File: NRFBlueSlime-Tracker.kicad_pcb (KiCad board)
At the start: 4 copper layers, 30 x 23.5 mm, 81 parts, among them J1 HC-TYPE-C-16P-C10B, Q1 YFW2301T, SW1 TS-1088-AR02016, U1 nRF52840, U2 NPM1100-QDAA-R, U3 ICM-45686, U4 LIS2MDL, X1 SX2M32.768KM20F30TNN, Y1 XL7EL89CKI-111YLC-32M

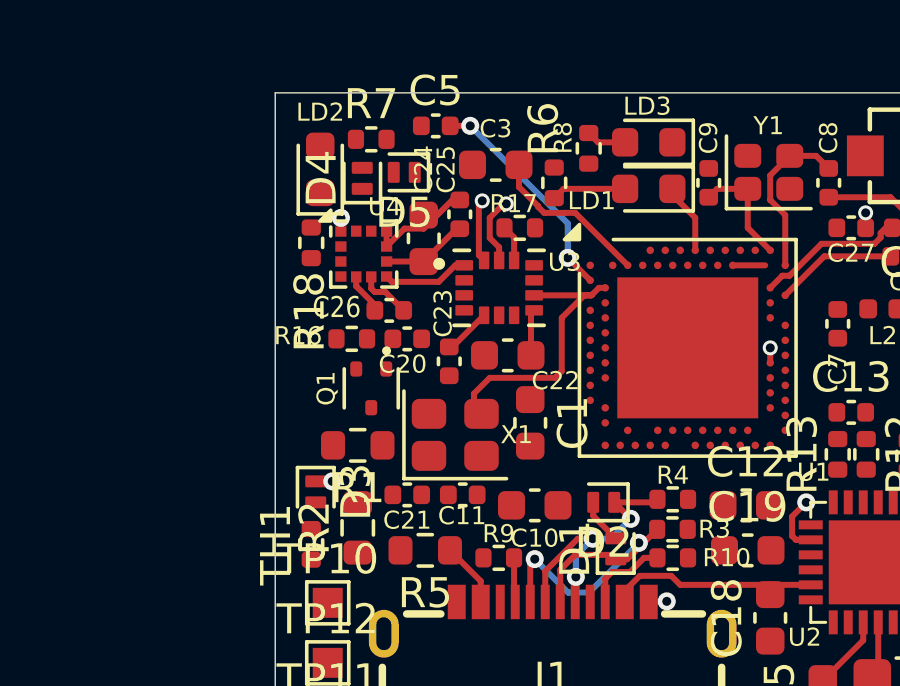
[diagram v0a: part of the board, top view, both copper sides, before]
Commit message: sync
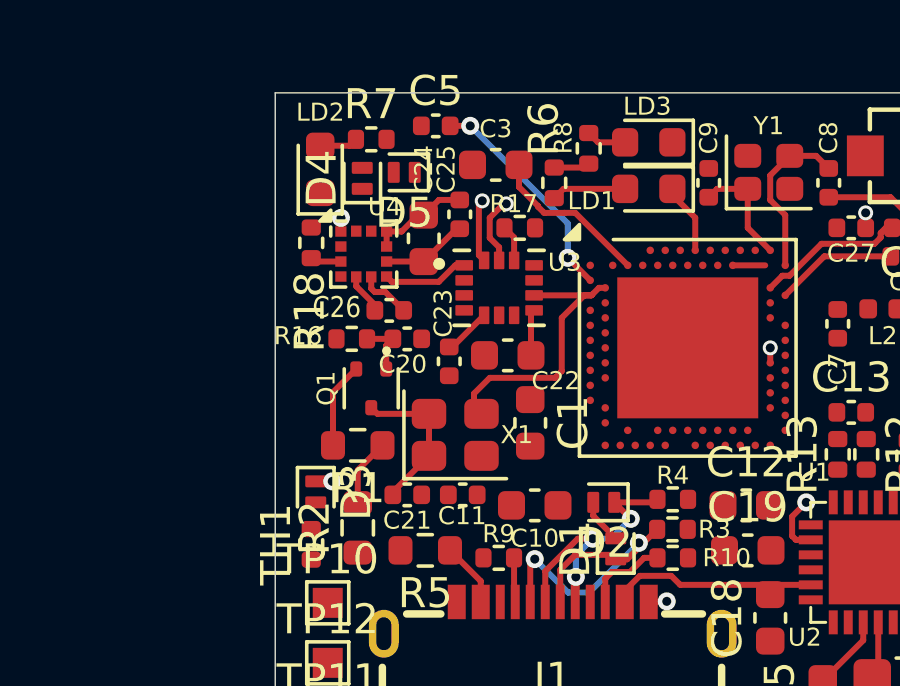
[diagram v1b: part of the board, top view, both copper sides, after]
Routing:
- net Net-(Q1-D): track 0.00 -> 5.21 mm
- net +1V8: track 10.4 -> 14.2 mm
- net Net-(U1-VDDH): track 0.00 -> 2.27 mm
- net ~{OSC_EN}: track 0.00 -> 1.96 mm
- net Net-(LD2-A): track 0.00 -> 1.28 mm
- net ~{CS}_MAG: track 0.00 -> 1.03 mm
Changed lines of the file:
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@@
+	)
+	(segment
+		(start 87.5625 47.1225)
+		(end 88.4375 47.1225)
+		(width 0.2)
+		(layer "F.Cu")
+		(net 21)
+	)
+	(segment
+		(start 87.45 47.01)
+		(end 87.5625 47.1225)
+		(width 0.2)
+		(layer "F.Cu")
+		(net 21)
 	)
 	(segment
@@
 	)
 	(segment
+		(start 92.4 45.07)
+		(end 91.705 45.07)
+		(width 0.2)
+		(layer "F.Cu")
+		(net 33)
+	)
+	(segment
 		(start 92.1575 49.97)
 		(end 93.2125 48.915)
@@
 	)
 	(segment
+		(start 96.57 43.99)
+		(end 96.7 43.86)
+		(width 0.2)
+		(layer "F.Cu")
+		(net 33)
+	)
+	(segment
 		(start 92.05 49.97)
 		(end 92.1575 49.97)
@@
 	)
 	(segment
+		(start 91.705 45.07)
+		(end 91.2 45.575)
+		(width 0.2)
+		(layer "F.Cu")
+		(net 33)
+	)
+	(segment
 		(start 89.9625 46.1225)
 		(end 89.9625 46.6225)
@@
 	)
 	(segment
-		(start 92.4 45.07)
-		(end 92.155 45.07)
-		(width 0.2)
-		(layer "F.Cu")
-		(net 33)
-	)
-	(segment
-		(start 92.155 45.07)
-		(end 91.2 46.025)
-		(width 0.2)
-		(layer "F.Cu")
-		(net 33)
-	)
-	(segment
 		(start 94.775 48.8525)
 		(end 94.8775 48.75)
@@
 	)
 	(segment
-		(start 90.56 46.025)
-		(end 89.9625 46.6225)
-		(width 0.2)
-		(layer "F.Cu")
-		(net 33)
-	)
-	(segment
-		(start 91.2 46.025)
-		(end 90.56 46.025)
+		(start 88.175 53.25)
+		(end 88.175 51.48)
+		(width 0.2)
+		(layer "F.Cu")
+		(net 33)
+	)
+	(segment
+		(start 95.55 43.99)
+		(end 96.57 43.99)
+		(width 0.2)
+		(layer "F.Cu")
+		(net 33)
+	)
+	(segment
+		(start 91.01 45.575)
+		(end 90.4625 46.1225)
+		(width 0.2)
+		(layer "F.Cu")
+		(net 33)
+	)
+	(segment
+		(start 91.2 45.575)
+		(end 91.01 45.575)
+		(width 0.2)
+		(layer "F.Cu")
+		(net 33)
+	)
+	(segment
+		(start 90.4625 46.1225)
+		(end 89.9625 46.1225)
 		(width 0.2)
 		(layer "F.Cu")
@@
 	)
 	(segment
+		(start 88.175 51.48)
+		(end 88.95 50.705)
+		(width 0.2)
+		(layer "F.Cu")
+		(net 33)
+	)
+	(segment
 		(start 101.61 64)
 		(end 101.13 63.52)
@@
 	)
 	(segment
+		(start 89.95 49.92)
+		(end 90.17 49.7)
+		(width 0.2)
+		(layer "F.Cu")
+		(net 38)
+	)
+	(segment
+		(start 89.95 50.705)
+		(end 89.95 49.92)
+		(width 0.2)
+		(layer "F.Cu")
+		(net 38)
+	)
+	(segment
+		(start 89.31 49.7)
+		(end 90.17 49.7)
+		(width 0.2)
+		(layer "F.Cu")
+		(net 38)
+	)
+	(segment
+		(start 91.375 52.2)
+		(end 89.655 52.2)
+		(width 0.2)
+		(layer "F.Cu")
+		(net 42)
+	)
+	(segment
+		(start 90.17 54.805)
+		(end 91.375 53.6)
+		(width 0.2)
+		(layer "F.Cu")
+		(net 42)
+	)
+	(segment
+		(start 90.17 54.9)
+		(end 90.17 54.805)
+		(width 0.2)
+		(layer "F.Cu")
+		(net 42)
+	)
+	(segment
+		(start 91.375 53.6)
+		(end 91.375 52.2)
+		(width 0.2)
+		(layer "F.Cu")
+		(net 42)
+	)
+	(segment
+		(start 89.655 52.2)
+		(end 89.45 51.995)
+		(width 0.2)
+		(layer "F.Cu")
+		(net 42)
+	)
+	(segment
 		(start 89.651822 48.65)
 		(end 88.95 47.948178)
@@
 	)
 	(segment
+		(start 88.7275 43.2625)
+		(end 88.94 43.05)
+		(width 0.2)
+		(layer "F.Cu")
+		(net 72)
+	)
+	(segment
+		(start 87.75 43.2625)
+		(end 88.7275 43.2625)
+		(width 0.2)
+		(layer "F.Cu")
+		(net 72)
+	)
+	(segment
 		(start 97.9125 43.15)
 		(end 97.01 43.15)
@@
 	)
 	(segment
+		(start 89 54.075)
+		(end 89.825 53.25)
+		(width 0.2)
+		(layer "F.Cu")
+		(net 75)
+	)
+	(segment
+		(start 89 55.175)
+		(end 89 54.075)
+		(width 0.2)
+		(layer "F.Cu")
+		(net 75)
+	)
+	(segment

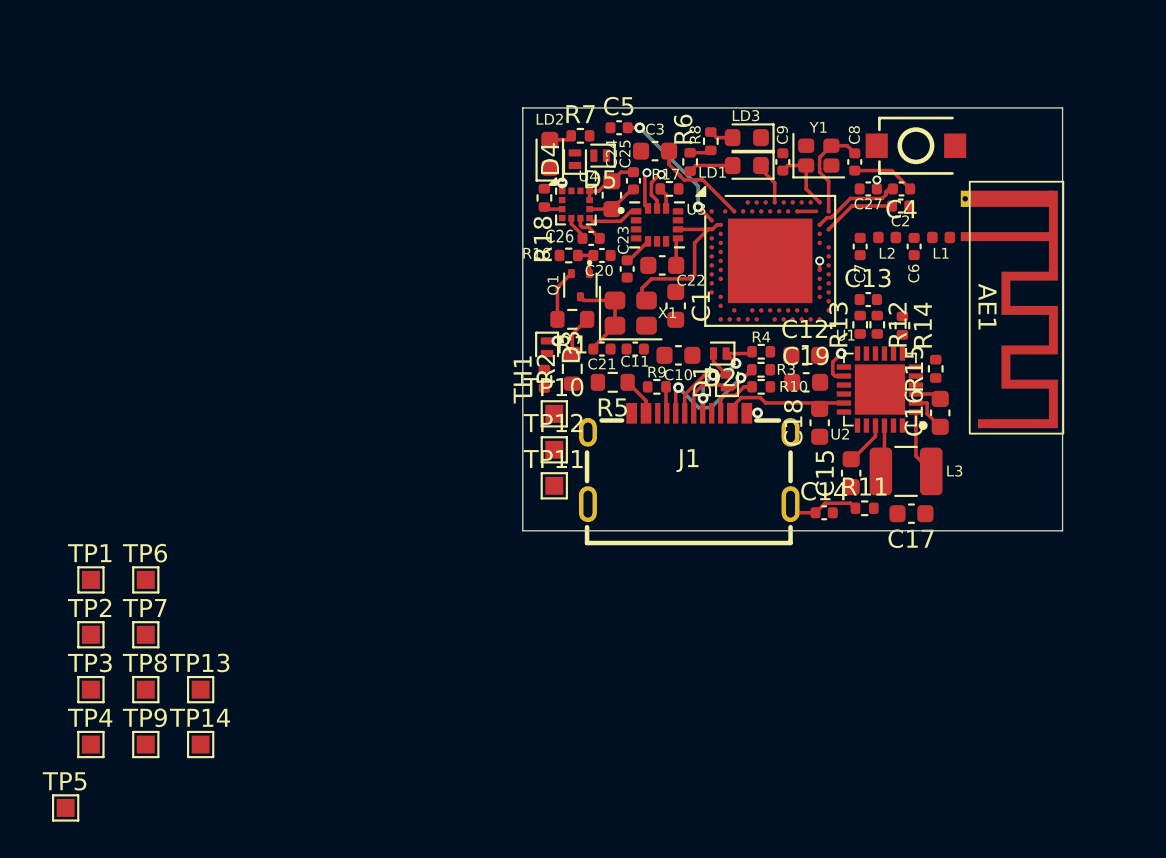
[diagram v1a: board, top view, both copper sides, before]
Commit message: sync
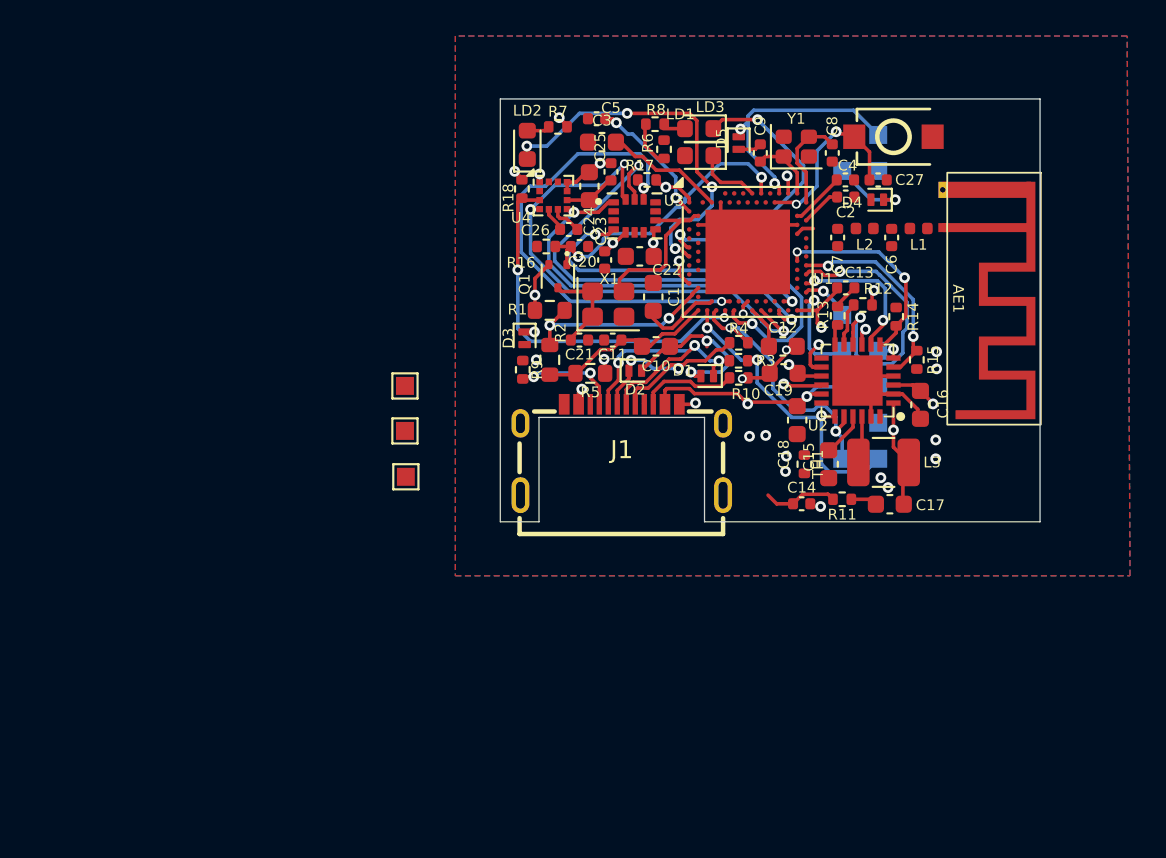
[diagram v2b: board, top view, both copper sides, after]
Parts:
- TP1, TP13, TP14, TP2, TP3, TP4, TP5, TP6, TP7, TP8, TP9: moved to B.Cu
- moved TP5 57.4 mm to (106.0, 45.0), turned to 180 degrees
- moved TP9 50.1 mm to (104.0, 45.0), turned to 180 degrees
- moved TP13 48.7 mm to (106.0, 43.0), turned to 180 degrees
- moved TP4 47.3 mm to (106.0, 59.0), turned to 180 degrees
- moved TP3 46.7 mm to (104.0, 53.0), turned to 180 degrees
- moved TP2 46.5 mm to (106.0, 55.0), turned to 180 degrees
- moved TP1 43.7 mm to (104.0, 55.0), turned to 180 degrees
- moved TP8 42.7 mm to (106.0, 61.0), turned to 180 degrees
- moved TP14 42.6 mm to (106.0, 57.0), turned to 180 degrees
- moved TP6 40.2 mm to (104.0, 57.0), turned to 180 degrees
- moved TP7 39.9 mm to (104.0, 61.0), turned to 180 degrees
- moved D4 16.9 mm to (106.0, 46.6), turned to 180 degrees
- moved TH1 15.2 mm to (101.9, 61.3), turned to -90 degrees
- moved TP10 8.44 mm to (79.7, 57.0)
- moved TP12 8.37 mm to (79.7, 59.5)
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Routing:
- net MOSI: track 2.10 -> 29.0 mm, vias 1 -> 3
- net ~{CS}_IMU: track 1.22 -> 26.8 mm, vias 0 -> 2
- net INT: track 0.00 -> 23.9 mm, vias 0 -> 2
- net SCLK: track 2.75 -> 24.6 mm, vias 2 -> 3
- net GND: track 12.7 -> 34.4 mm, vias 1 -> 17
- net VBUS: track 8.88 -> 30.5 mm, vias 1 -> 5
- net ~{LED_ERR}: track 0.00 -> 21.2 mm, vias 0 -> 4
- net ~{CS}_MAG: track 1.03 -> 21.1 mm, vias 0 -> 2
- net MISO: track 2.89 -> 22.1 mm, vias 0 -> 2
- net DN: track 0.00 -> 17.8 mm, vias 0 -> 3
- net ~{RST}: track 0.00 -> 17.8 mm, vias 0 -> 2
- net ~{LED_CHG}: track 0.00 -> 16.5 mm, vias 0 -> 2
- net NPM_~{ERR}: track 0.00 -> 16.4 mm, vias 0 -> 2
- net +1V8: track 14.2 -> 30.4 mm, vias 0 -> 11
- net VSYS: track 1.46 -> 17.5 mm, vias 0 -> 3
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- added copper zone on In1.Cu, net +1V8
- added copper zone on B.Cu, net GND
- added copper zone on F.Cu, net GND
- added copper zone on In2.Cu, net GND
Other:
- outline, holes or cut-outs redrawn
